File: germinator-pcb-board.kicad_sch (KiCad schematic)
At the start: 10 parts, among them J1 Conn_01x15_Socket, J2 Conn_01x15_Socket, J3 Screw_Terminal_01x04, J4 Screw_Terminal_01x03, J5 Screw_Terminal_01x03, J6 Screw_Terminal_01x03, J7 Screw_Terminal_01x03, U1 ESP32-DEVKIT-V1

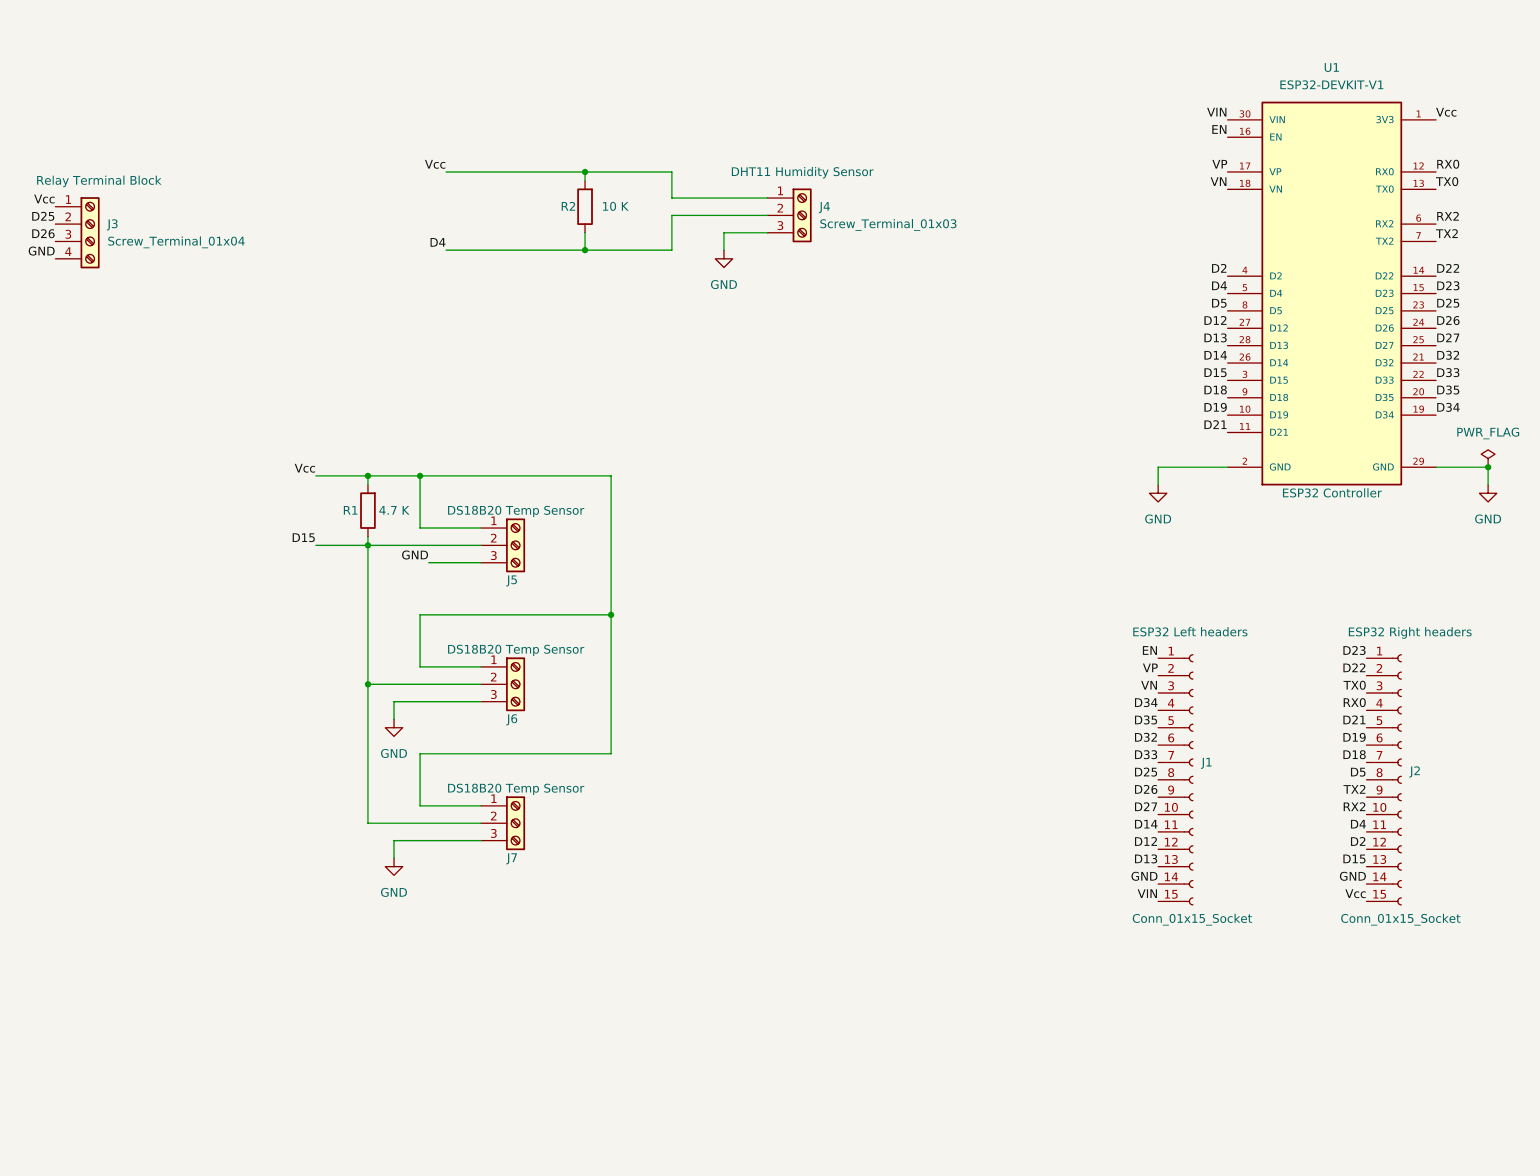
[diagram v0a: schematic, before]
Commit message: Schematics step 7: Comments
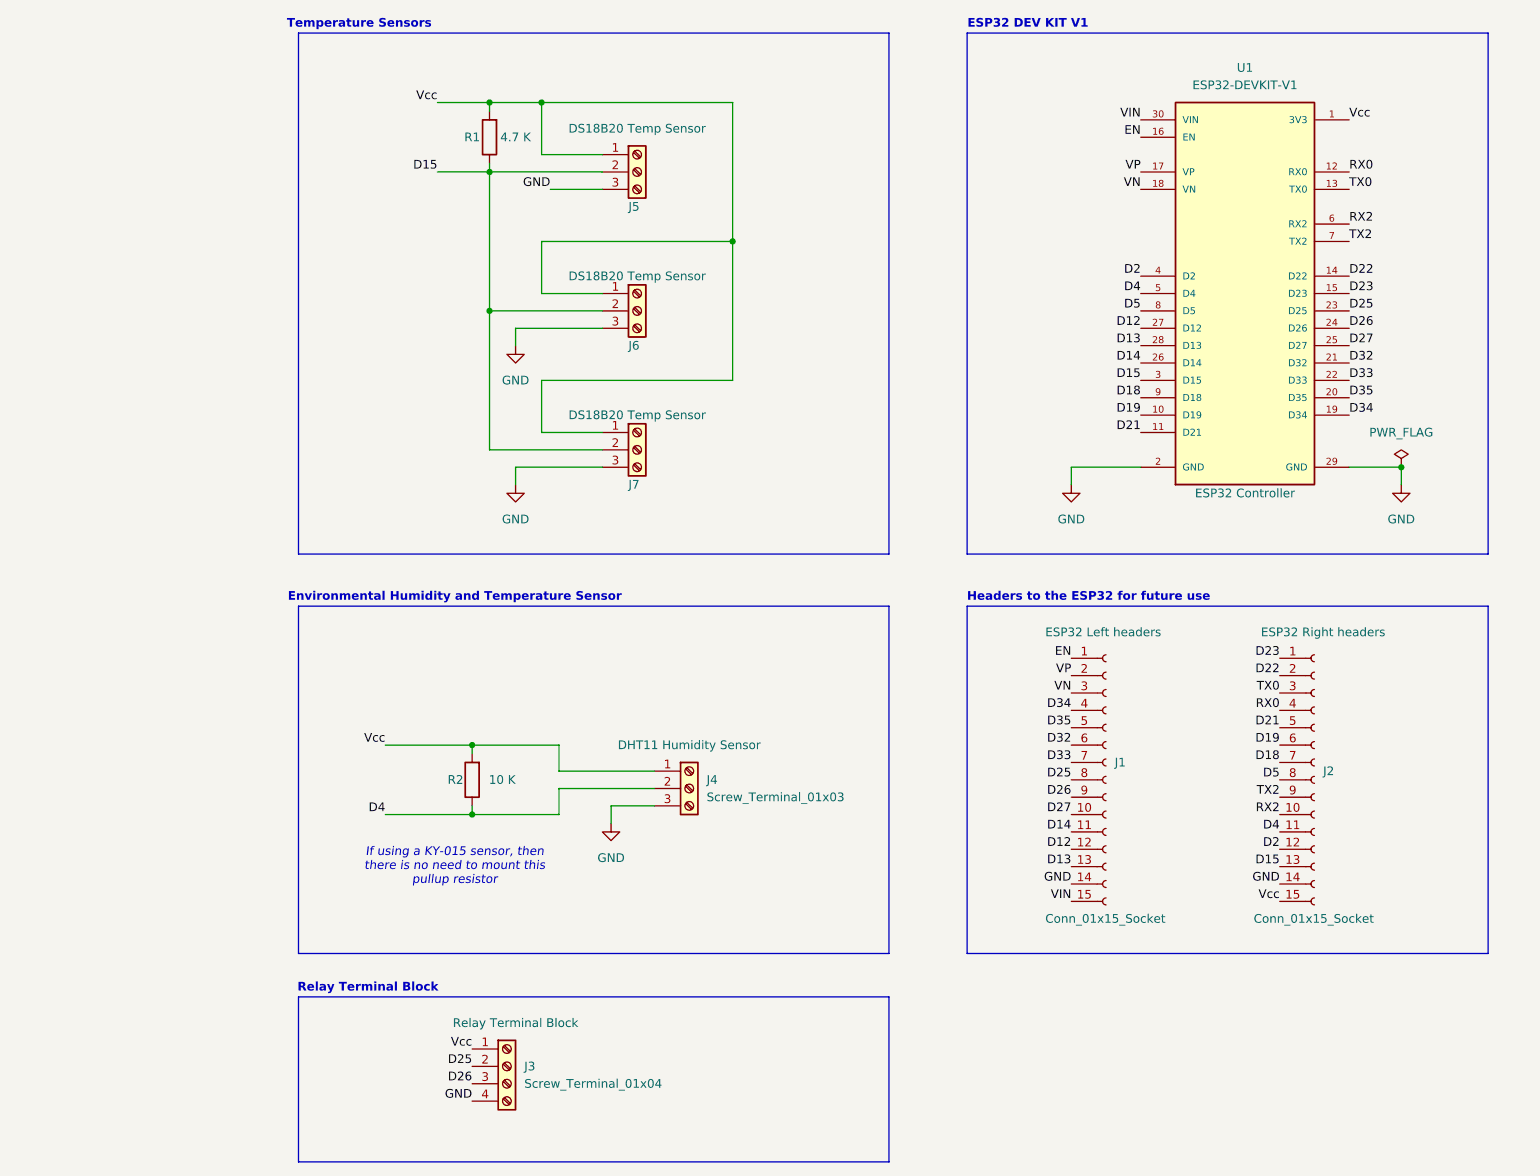
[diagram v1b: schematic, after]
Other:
- note added: "ESP32 DEV KIT V1"
- note added: "Environmental Humidity and Temperature Sensor"
- note added: "Headers to the ESP32 for future use"
- note added: "If using a KY-015 sensor, then there is no need to mount this pullup resistor"
- note added: "Relay Terminal Block"
- note added: "Temperature Sensors"
- moved on the sheet: J1, J2, J3, J4, J5, J6, J7, R1, R2, U1
